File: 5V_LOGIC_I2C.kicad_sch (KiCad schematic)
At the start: 10 parts, among them J601 2350514-8, J602 XH-4A connector, U601 TLA2528IRTER

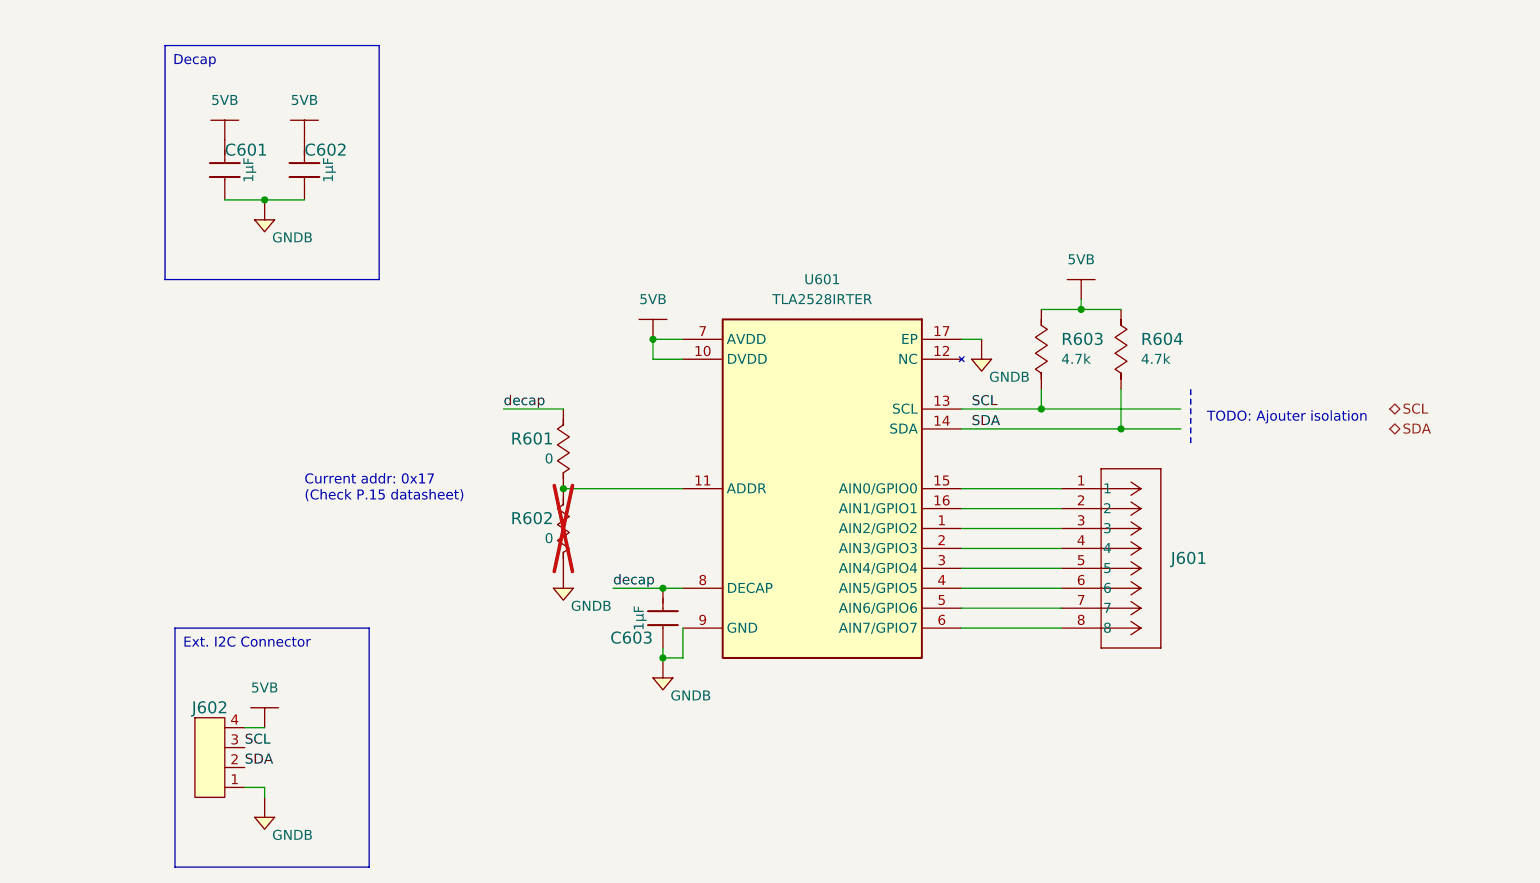
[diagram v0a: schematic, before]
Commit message: modif schématique
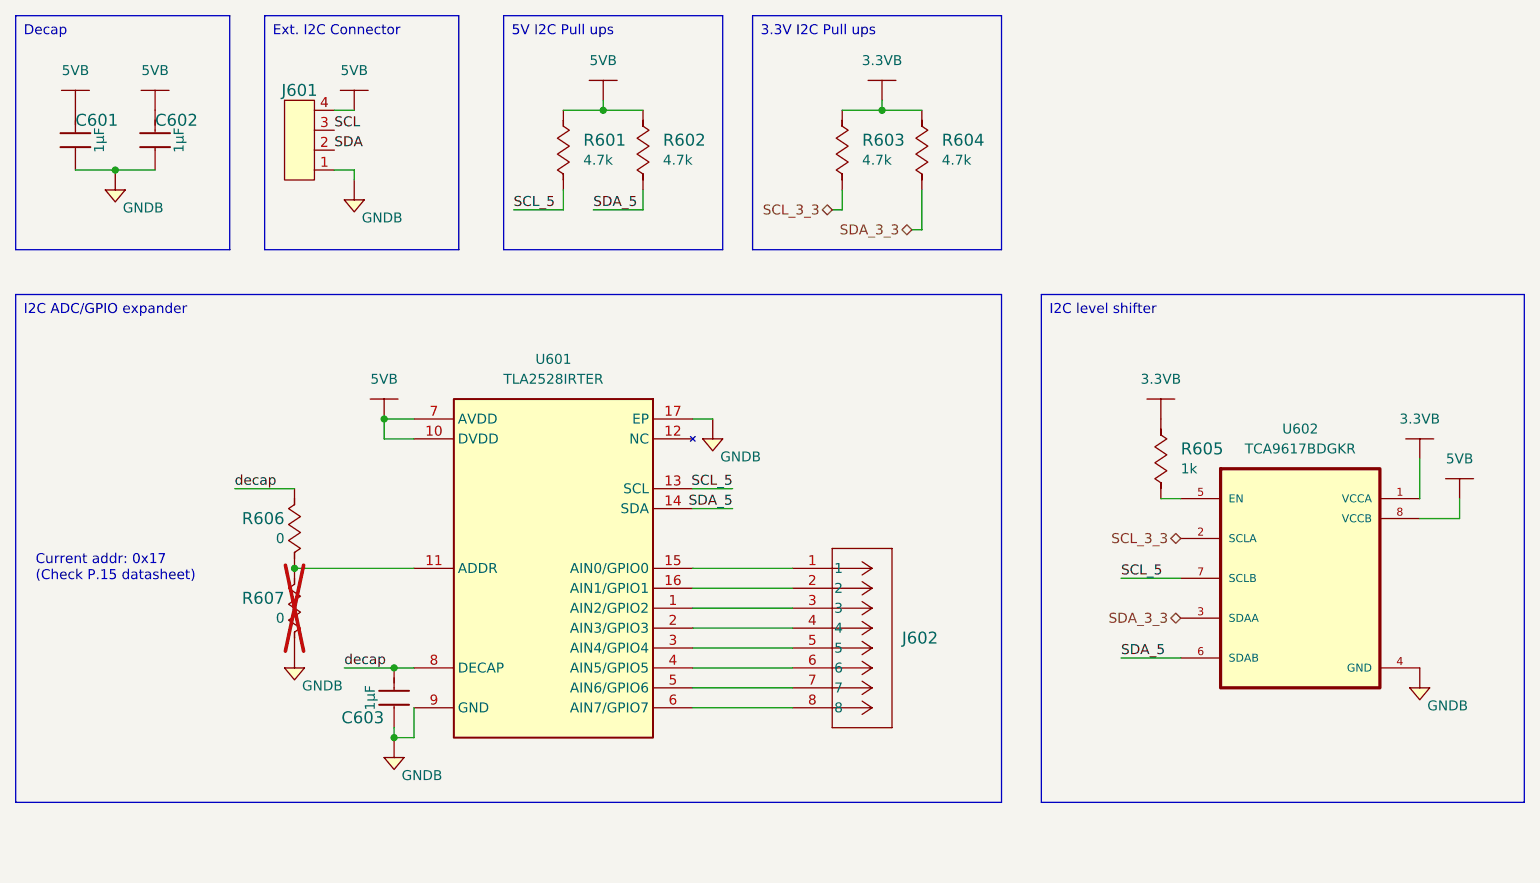
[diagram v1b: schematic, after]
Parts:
- added R603, R604: RC0805JR-074K7L, Resistors:R0805, symbol Resistors:RC0805JR-074K7L
- added R605: RC0805JR-071KL, Resistors:R0805, symbol Resistors:RC0805JR-071KL
- added U602: TCA9617BDGKR, IC:SOP65P490X110-8N, symbol Interface:TCA9617BDGKR
- renumbered J602 to J601, J601 to J602, R603 to R601, R604 to R602, R601 to R606, R602 to R607
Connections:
- net 5VB: now also U602.8 (VCCB)
- net GNDB: now also U602.4 (GND)
- net SCL: no longer R601.1, U601.13 (SCL)
- net SDA: no longer R602.1, U601.14 (SDA)
- new net: R605.2, U602.5 (EN)
- new net 3.3VB: R603.2, R604.2, R605.1, U602.1 (VCCA)
- new net SCL_3_3: R603.1, U602.2 (SCLA)
- new net SCL_5: R601.1, U601.13 (SCL), U602.7 (SCLB)
- new net SDA_3_3: R604.1, U602.3 (SDAA)
- new net SDA_5: R602.1, U601.14 (SDA), U602.6 (SDAB)
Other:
- note removed: "TODO: Ajouter isolation"
- title: (none) -> 5V Logic I2C
- moved on the sheet: C601, C602, C603, J601, J602, R601, R602, R606, R607, U601
